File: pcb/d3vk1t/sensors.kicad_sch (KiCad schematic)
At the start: 3 parts, among them IC1 LSM6DSMTR, IC2 HDC1080DMBR, IC3 LPS22HBTR

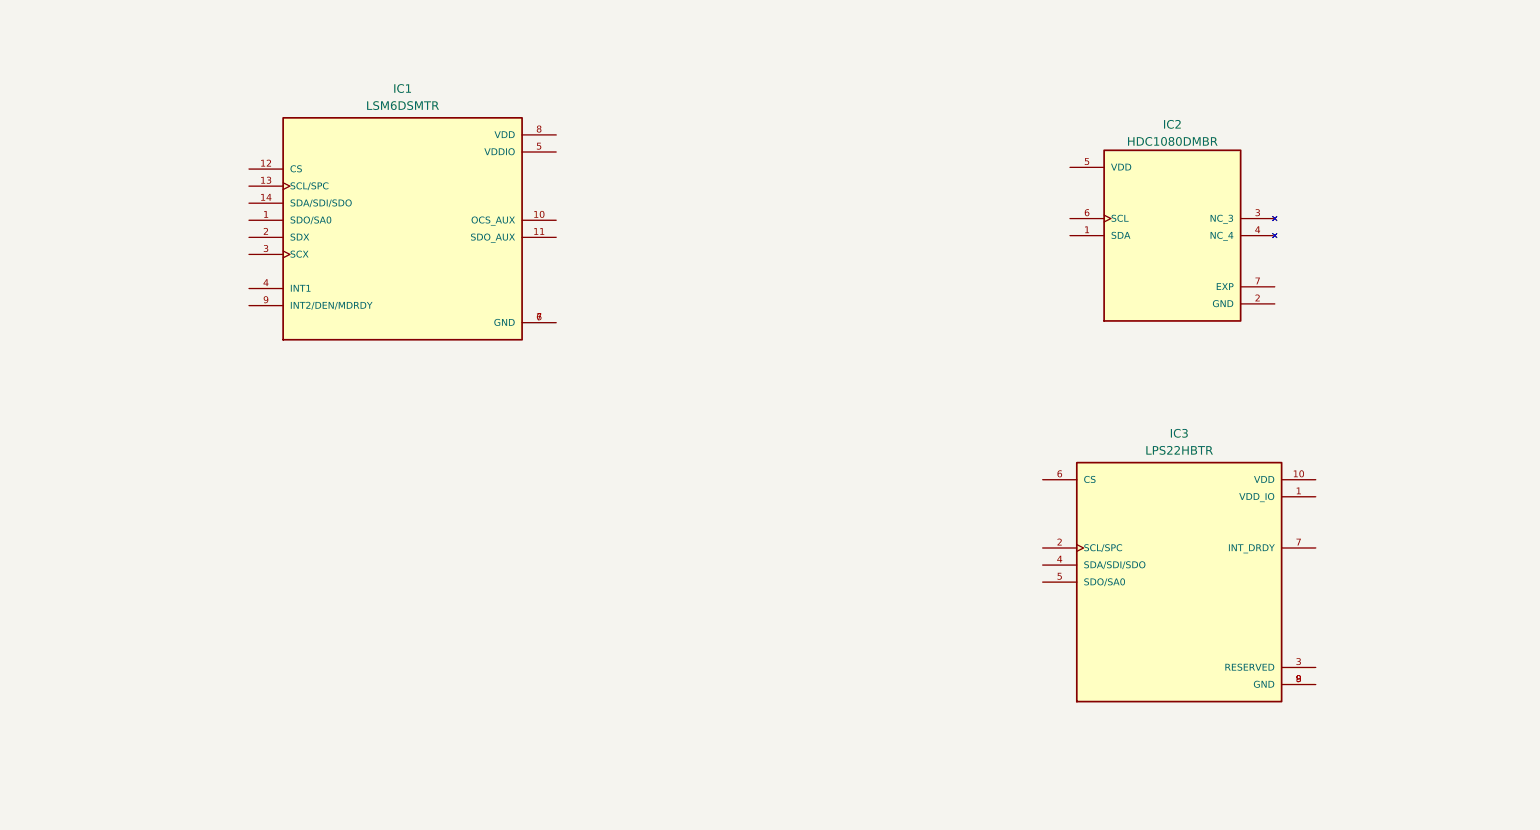
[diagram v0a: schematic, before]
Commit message: [update all schematics sheets]
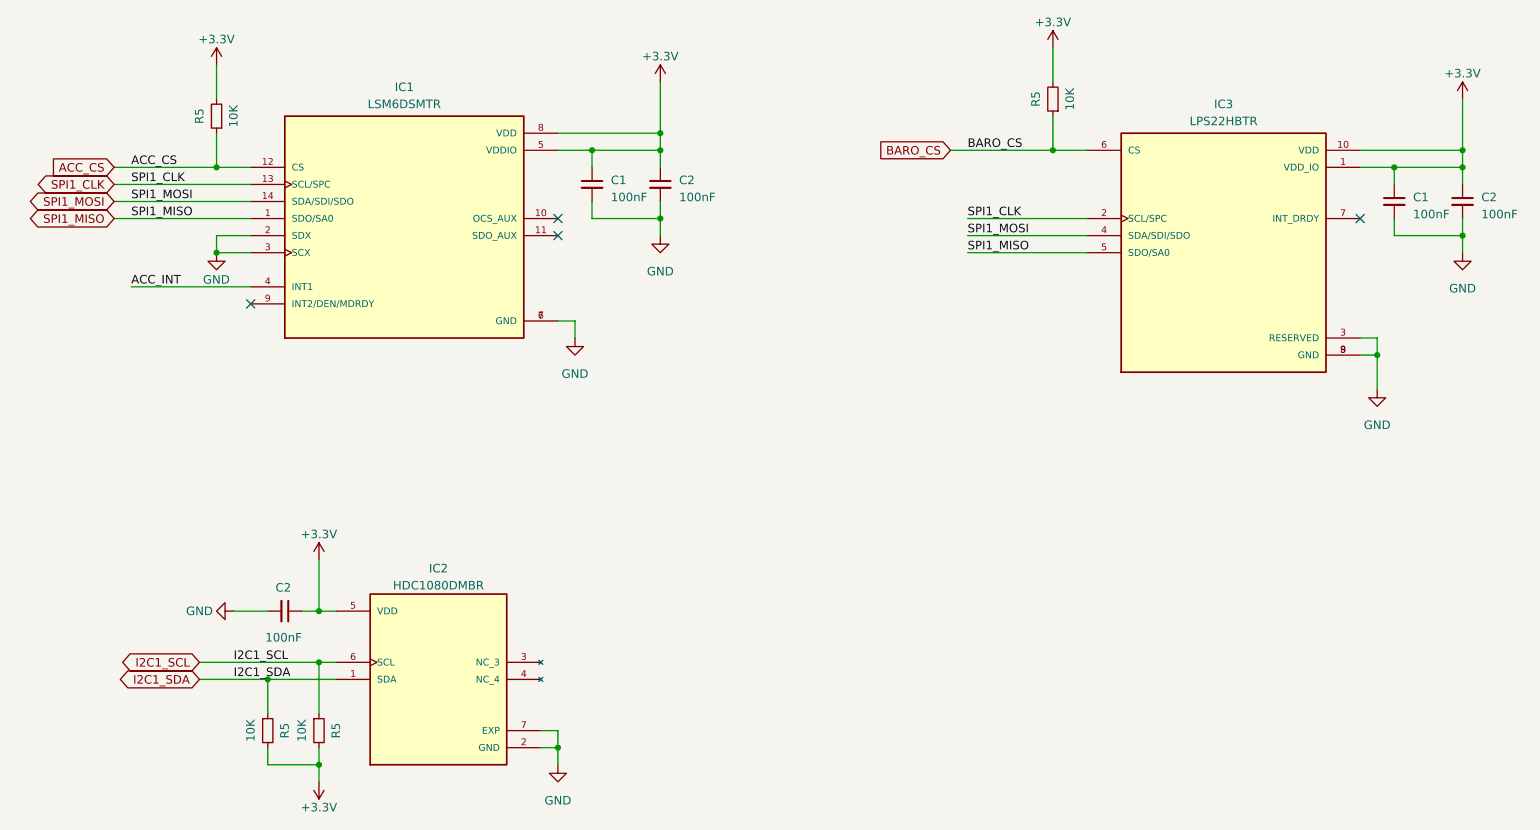
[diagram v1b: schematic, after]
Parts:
- added C1 (x2), C2 (x3): 100nF, Capacitor_SMD:C_0402_1005Metric, symbol Device:C_Small
- added R5 (x4): 10K, Resistor_SMD:R_0402_1005Metric, symbol Device:R_Small
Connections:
- net SPI1_MISO: now reaches IC1.1 (SDO/SA0)
- net SPI1_MISO: now also IC3.5 (SDO/SA0)
- net ACC_CS: now reaches IC1.12 (CS)
- net ACC_CS: now also R5.1
- net SPI1_CLK: now reaches IC1.13 (SCL/SPC)
- net SPI1_CLK: now also IC3.2 (SCL/SPC)
- net SPI1_MOSI: now reaches IC1.14 (SDA/SDI/SDO)
- net SPI1_MOSI: now also IC3.4 (SDA/SDI/SDO)
- net GND: now reaches IC1.2 (SDX)
- net GND: now also IC1.3 (SCX), IC1.6 (GND), IC1.7 (GND), IC2.2 (GND), IC2.7 (EXP), IC3.3 (RESERVED), IC3.8 (GND), IC3.9 (GND), C1.2, C1.2, C2.2, C2.2, C2.2
- net ACC_INT: now reaches IC1.4 (INT1)
- net +3.3V: now reaches IC1.5 (VDDIO)
- net +3.3V: now also IC1.8 (VDD), IC2.5 (VDD), IC3.1 (VDD_IO), IC3.10 (VDD), C1.1, C1.1, C2.1, C2.1, C2.1, R5.2, R5.2, R5.2, R5.2
- net BARO_CS: now reaches IC3.6 (CS)
- net BARO_CS: now also R5.1
- net I2C1_SDA: now reaches IC2.1 (SDA)
- net I2C1_SDA: now also R5.1
- net I2C1_SCL: now reaches IC2.6 (SCL)
- net I2C1_SCL: now also R5.1
- no-connect marks 0 -> 4
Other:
- moved on the sheet: IC2, IC3
